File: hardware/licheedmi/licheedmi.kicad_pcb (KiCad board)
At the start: 4 copper layers, 94 x 38 mm, 75 parts, among them J1 Conn_01x09, J2 HDMI_A_PCB, J3 LicheePiNano_LCD, J4 HDMI_A, J5 USB_C_Receptacle_USB2.0, U1 TDA19988, U2 LicheeNano, U3 TS3DV20812, U4 SC6206B, U5 CH340C

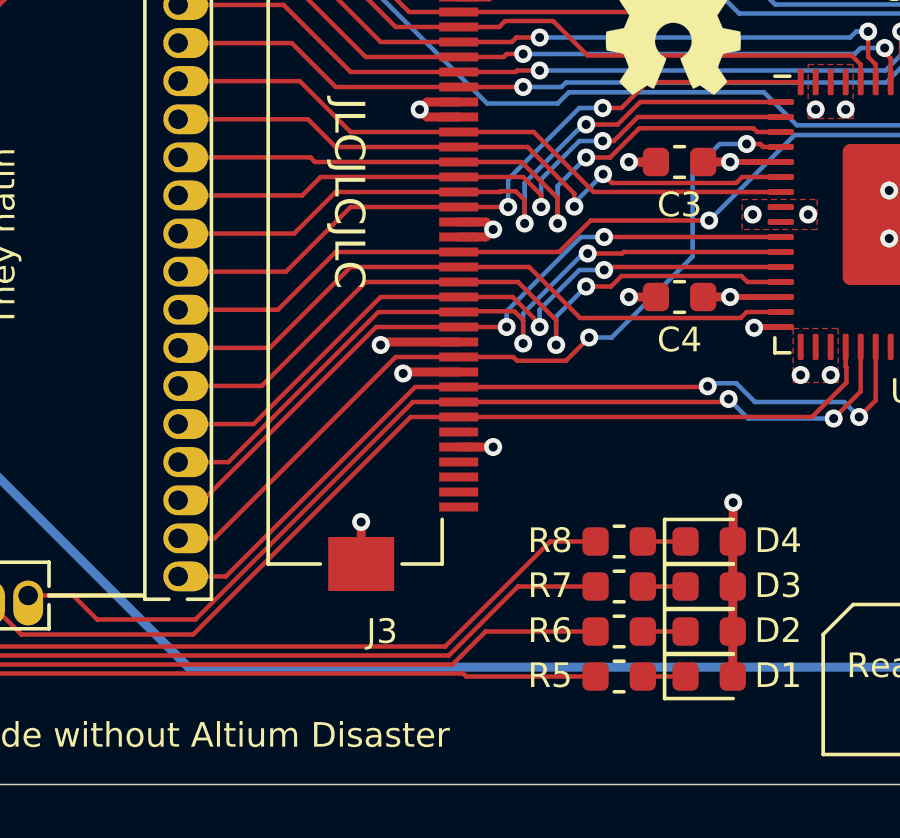
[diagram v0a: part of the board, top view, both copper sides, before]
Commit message: Add FPC connector 3D model
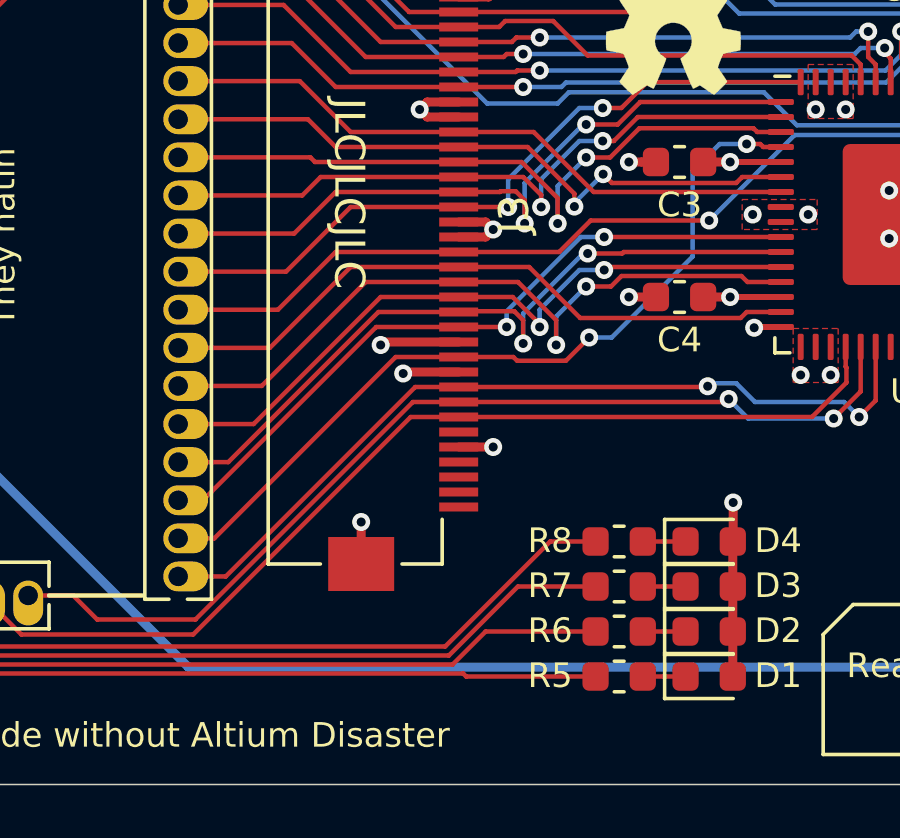
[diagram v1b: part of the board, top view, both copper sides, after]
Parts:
- J3: footprint Connector_FFC-FPC:Hirose_FH12-40S-0.5SH_1x40-1MP_P0.50mm_Horizontal -> hdmizness:Hirose_FH12-40S-0.5SH_1x40-1MP_P0.50mm_Horizontal
